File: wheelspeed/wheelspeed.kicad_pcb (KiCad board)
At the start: 2 copper layers, 20 x 18.5 mm, 12 parts, among them J1 Conn_01x04_Pin, U1 TMAG5111B2xxDBV

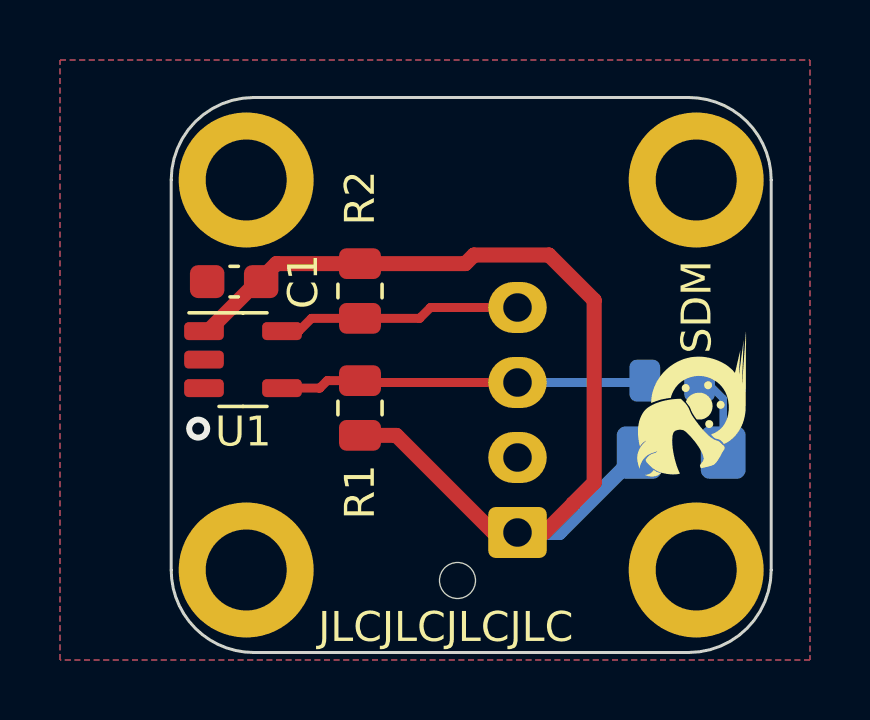
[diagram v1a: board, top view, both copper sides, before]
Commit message: logger updates
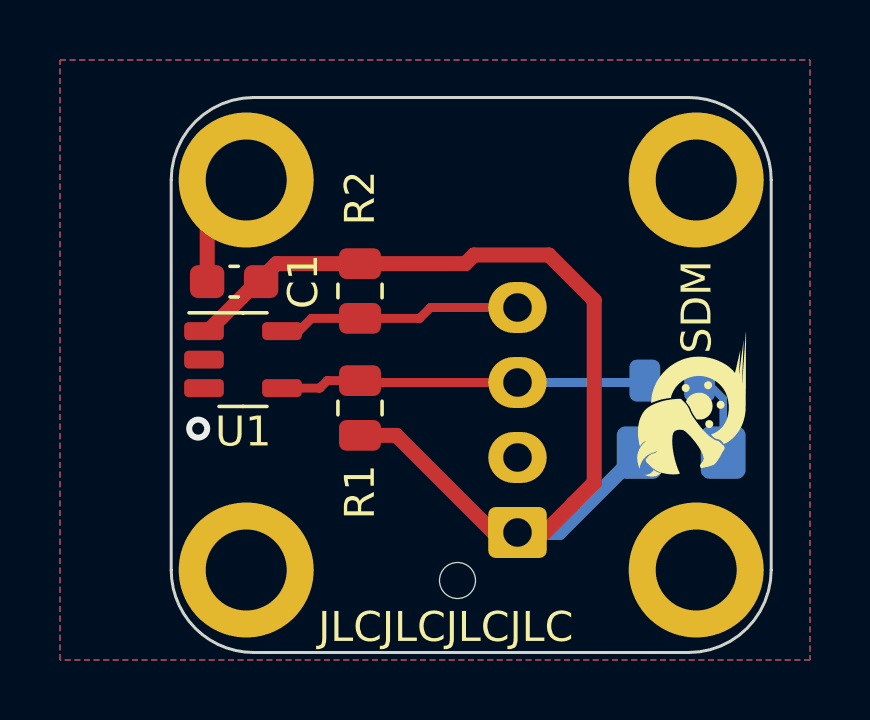
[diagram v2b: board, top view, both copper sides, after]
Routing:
- net GND: track 0.00 -> 3.93 mm
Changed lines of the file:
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@@
   (segment (start 142.9375 102.1625) (end 145.6 99.5) (width 0.5) (layer "B.Cu") (net 1))
   (segment (start 141.54375 102.1625) (end 142.9375 102.1625) (width 0.5) (layer "B.Cu") (net 1))
+  (segment (start 131.2 91.7125) (end 132.5 90.4125) (width 0.5) (layer "F.Cu") (net 2))
+  (segment (start 131.2 93.8) (end 131.2 91.7125) (width 0.5) (layer "F.Cu") (net 2))
   (via (at 130.9 98.7) (size 0.8) (drill 0.4) (layers "F.Cu" "B.Cu") (free) (net 2))
   (segment (start 141.54375 97.1625) (end 136.35625 97.1625) (width 0.3) (layer "F.Cu") (net 3))

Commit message: fahb files
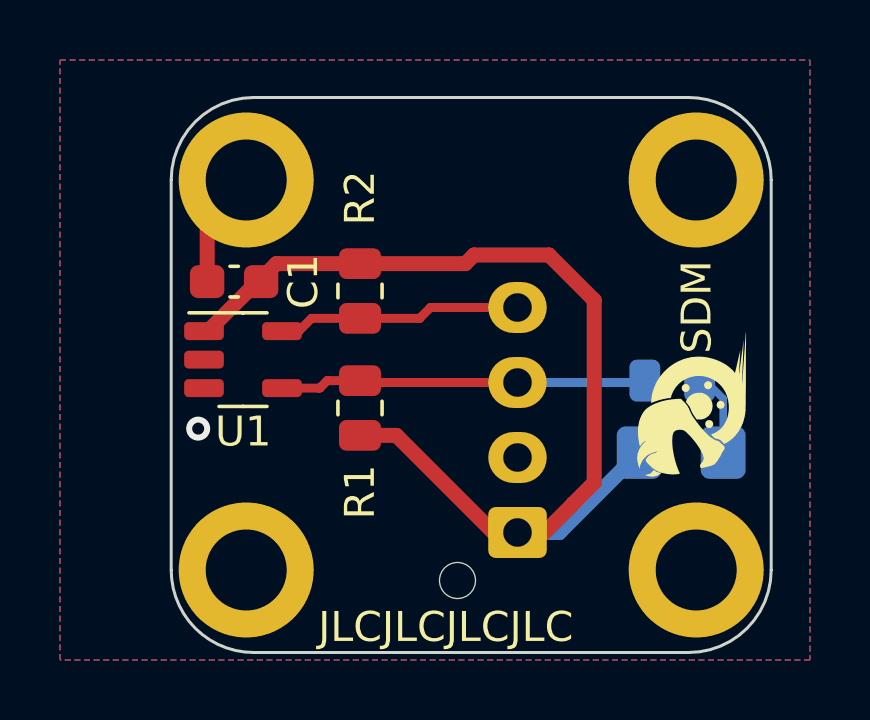
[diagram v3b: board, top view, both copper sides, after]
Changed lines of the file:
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@@
       (plot_on_all_layers_selection 0x0000000_00000000)
       (disableapertmacros false)
-      (usegerberextensions false)
-      (usegerberattributes true)
-      (usegerberadvancedattributes true)
-      (creategerberjobfile true)
+      (usegerberextensions true)
+      (usegerberattributes false)
+      (usegerberadvancedattributes false)
+      (creategerberjobfile false)
       (dashed_line_dash_ratio 12.000000)
       (dashed_line_gap_ratio 3.000000)
@@
       (psa4output false)
       (plotreference true)
-      (plotvalue true)
+      (plotvalue false)
       (plotinvisibletext false)
       (sketchpadsonfab false)
-      (subtractmaskfromsilk false)
+      (subtractmaskfromsilk true)
       (outputformat 1)
       (mirror false)
-      (drillshape 1)
+      (drillshape 0)
       (scaleselection 1)
-      (outputdirectory "")
+      (outputdirectory "fab/")
     )
   )
@@
     (fp_line (start 1 0.625) (end -1 0.625)
       (stroke (width 0.1) (type solid)) (layer "F.Fab"))
-    (pad "1" smd roundrect (at -0.9125 0 270) (size 1.025 1.4) (layers "F.Cu" "F.Paste" "F.Mask") (roundrect_rratio 0.243902)
+    (pad "1" smd roundrect (at -0.9125 0 270) (size 1.025 1.4) (layers "F.Cu" "F.Paste" "F.Mask") (roundrect_rratio 0.243902439)
       (net 1 "VCC") (pintype "passive"))
-    (pad "2" smd roundrect (at 0.9125 0 270) (size 1.025 1.4) (layers "F.Cu" "F.Paste" "F.Mask") (roundrect_rratio 0.243902)
+    (pad "2" smd roundrect (at 0.9125 0 270) (size 1.025 1.4) (layers "F.Cu" "F.Paste" "F.Mask") (roundrect_rratio 0.243902439)
       (net 4 "/DIR") (pintype "passive"))
     (model "${KICAD6_3DMODEL_DIR}/Resistor_SMD.3dshapes/R_0805_2012Metric.wrl"
@@
     (fp_line (start 1 0.625) (end -1 0.625)
       (stroke (width 0.1) (type solid)) (layer "F.Fab"))
-    (pad "1" smd roundrect (at -0.9125 0 90) (size 1.025 1.4) (layers "F.Cu" "F.Paste" "F.Mask") (roundrect_rratio 0.243902)
+    (pad "1" smd roundrect (at -0.9125 0 90) (size 1.025 1.4) (layers "F.Cu" "F.Paste" "F.Mask") (roundrect_rratio 0.243902439)
       (net 1 "VCC") (pintype "passive"))
-    (pad "2" smd roundrect (at 0.9125 0 90) (size 1.025 1.4) (layers "F.Cu" "F.Paste" "F.Mask") (roundrect_rratio 0.243902)
+    (pad "2" smd roundrect (at 0.9125 0 90) (size 1.025 1.4) (layers "F.Cu" "F.Paste" "F.Mask") (roundrect_rratio 0.243902439)
       (net 3 "/SPEED") (pintype "passive"))
     (model "${KICAD6_3DMODEL_DIR}/Resistor_SMD.3dshapes/R_0805_2012Metric.wrl"
@@
       (stroke (width 0.1) (type solid)) (layer "B.Fab"))
     (pad "" np_thru_hole circle (at -1.6 -2 90) (size 1.2 1.2) (drill 1.2) (layers "*.Cu" "*.Mask"))
-    (pad "1" thru_hole roundrect (at 0 0 90) (size 1.7 1.95) (drill 0.95) (layers "*.Cu" "*.Mask") (roundrect_rratio 0.147059)
+    (pad "1" thru_hole roundrect (at 0 0 90) (size 1.7 1.95) (drill 0.95) (layers "*.Cu" "*.Mask") (roundrect_rratio 0.1470588235)
       (net 1 "VCC") (pinfunction "Pin_1") (pintype "passive"))
     (pad "2" thru_hole oval (at 2.5 0 90) (size 1.7 1.95) (drill 0.95) (layers "*.Cu" "*.Mask")
@@
     (fp_line (start 1 0.625) (end 1 -0.625)
       (stroke (width 0.1) (type solid)) (layer "B.Fab"))
-    (pad "1" smd roundrect (at -0.9125 0 180) (size 1.025 1.4) (layers "B.Cu" "B.Paste" "B.Mask") (roundrect_rratio 0.243902)
+    (pad "1" smd roundrect (at -0.9125 0 180) (size 1.025 1.4) (layers "B.Cu" "B.Paste" "B.Mask") (roundrect_rratio 0.243902439)
       (net 5 "/HE_LED") (pintype "passive"))
-    (pad "2" smd roundrect (at 0.9125 0 180) (size 1.025 1.4) (layers "B.Cu" "B.Paste" "B.Mask") (roundrect_rratio 0.243902)
+    (pad "2" smd roundrect (at 0.9125 0 180) (size 1.025 1.4) (layers "B.Cu" "B.Paste" "B.Mask") (roundrect_rratio 0.243902439)
       (net 3 "/SPEED") (pintype "passive"))
     (model "${KICAD6_3DMODEL_DIR}/Resistor_SMD.3dshapes/R_0805_2012Metric.wrl"
